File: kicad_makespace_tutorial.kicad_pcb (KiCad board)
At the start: 2 copper layers, 64.5 x 22.5 mm, 42 parts, among them J1 Screw_Terminal_01x02, J2 Conn_01x08_Pin, SW1 TS-1187A-B-A-B, SW2 TS-1187A-B-A-B, U1 AMS1117-3.3, U2 CH340C_C7464026, U3 ESP32-WROOM-32E(8MB), U4 MAX98357AETE+T

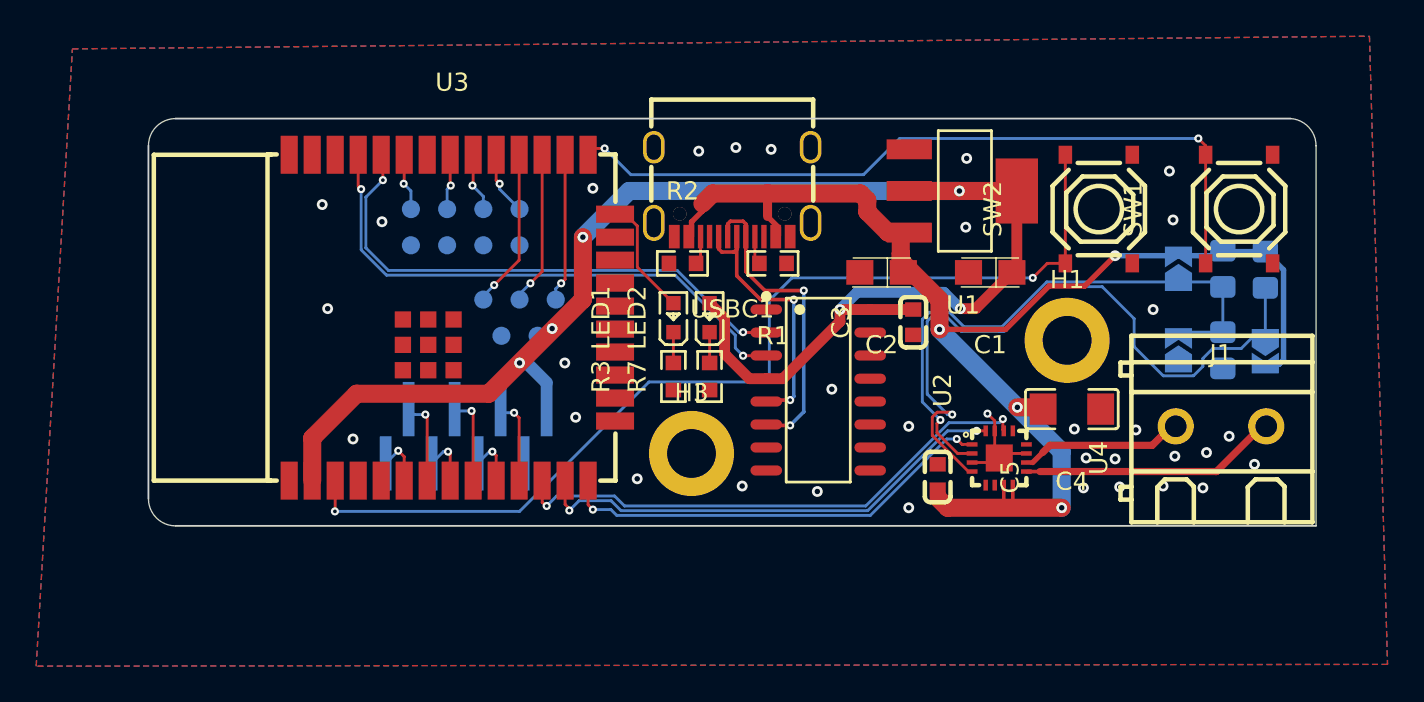
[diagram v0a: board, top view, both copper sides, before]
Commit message: Last updates
Signed-off-by: Pablo Garrido <pablogs9@gmail.com>
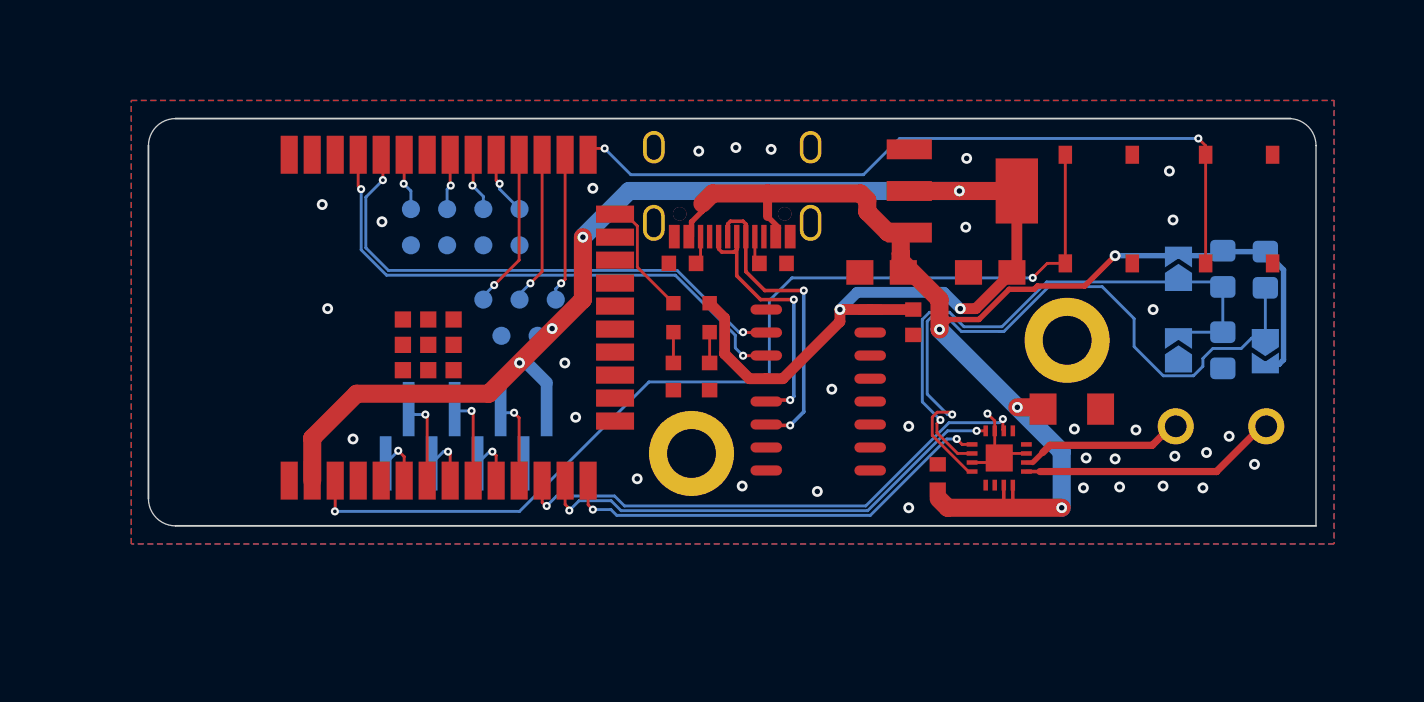
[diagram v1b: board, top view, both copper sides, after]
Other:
- board text added: "0"
- board text added: "0 mm"
- board text added: "0,01 mm"
- board text added: "0,02"
- board text added: "0,035 mm"
- board text added: "0,1600 mm / 0,1000 mm"
- board text added: "0,2000 mm"
- board text added: "1"
- board text added: "1 mm"
- board text added: "1,0900 mm"
- board text added: "2"
- board text added: "3,3"
- board text added: "4,5"
- board text added: "64,5000 mm x 22,5000 mm"
- board text added: "B.Cu"
- board text added: "B.Mask"
- board text added: "B.Paste"
- board text added: "B.Silkscreen"
- board text added: "BOARD CHARACTERISTICS"
- board text added: "Board Thickness:"
- board text added: "Board overall dimensions:"
- board text added: "Bottom Silk Screen"
- board text added: "Bottom Solder Mask"
- board text added: "Bottom Solder Paste"
- board text added: "Castellated pads:"
- board text added: "Color"
- board text added: "Copper Finish:"
- board text added: "Copper Layer Count:"
- board text added: "Dielectric 1"
- board text added: "Edge card connectors:"
- board text added: "Epsilon R"
- board text added: "F.Cu"
- board text added: "F.Mask"
- board text added: "F.Paste"
- board text added: "F.Silkscreen"
- board text added: "FR4"
- board text added: "Impedance Control:"
- board text added: "Layer Name"
- board text added: "Loss Tangent"
- board text added: "Material"
- board text added: "Min hole diameter:"
- board text added: "Min track/spacing:"
- board text added: "No"
- board text added: "None"
- board text added: "Not specified"
- board text added: "Plated Board Edge:"
- board text added: "Thickness (mm)"
- board text added: "Top Silk Screen"
- board text added: "Top Solder Mask"
- board text added: "Top Solder Paste"
- board text added: "Type"
- board text added: "copper"
- board text added: "core"

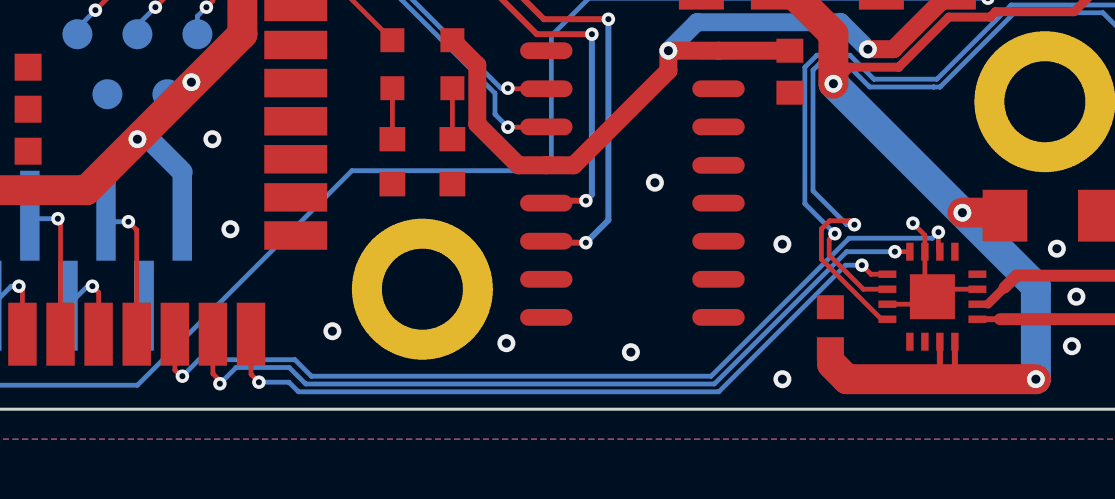
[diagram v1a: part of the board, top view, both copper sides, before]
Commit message: Minors
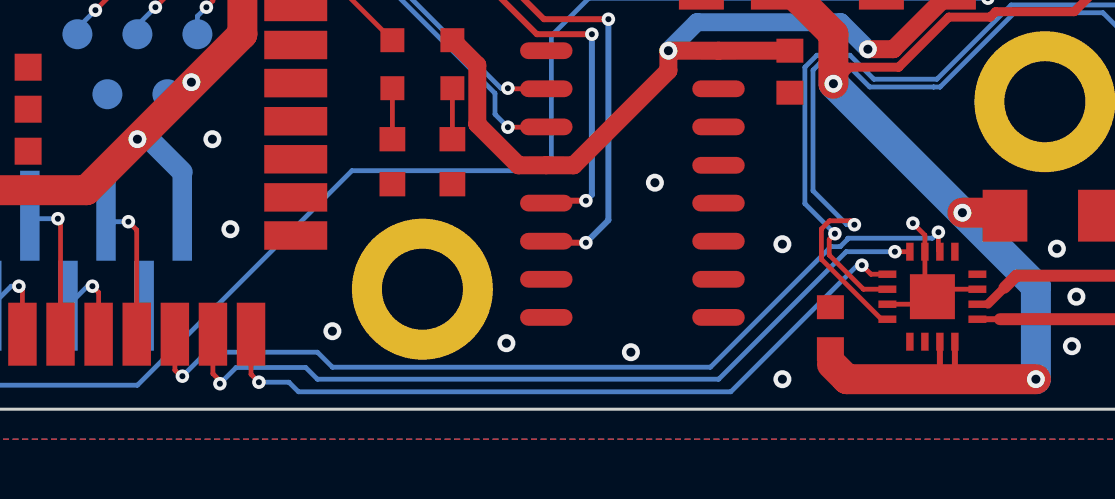
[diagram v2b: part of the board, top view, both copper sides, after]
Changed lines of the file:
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@@
-	)
-	(segment
-		(start 101.110001 121.660001)
-		(end 114.731887 121.660001)
-		(width 0.16)
-		(layer "B.Cu")
-		(net 36)
-	)
-	(segment
-		(start 119.141888 117.25)
-		(end 120.75 117.25)
-		(width 0.16)
-		(layer "B.Cu")
-		(net 36)
-	)
-	(segment
-		(start 98.79 121.11)
-		(end 100.56 121.11)
-		(width 0.16)
-		(layer "B.Cu")
-		(net 36)
-	)
-	(segment
-		(start 100.56 121.11)
-		(end 101.110001 121.660001)
-		(width 0.16)
-		(layer "B.Cu")
-		(net 36)
 	)
 	(segment
@@
 	)
 	(segment
-		(start 114.731887 121.660001)
-		(end 119.141888 117.25)
+		(start 114.875808 121.5)
+		(end 119.125808 117.25)
+		(width 0.16)
+		(layer "B.Cu")
+		(net 36)
+	)
+	(segment
+		(start 101.5 121.5)
+		(end 114.875808 121.5)
+		(width 0.16)
+		(layer "B.Cu")
+		(net 36)
+	)
+	(segment
+		(start 101.11 121.11)
+		(end 101.5 121.5)
+		(width 0.16)
+		(layer "B.Cu")
+		(net 36)
+	)
+	(segment
+		(start 119.125808 117.25)
+		(end 120.75 117.25)
+		(width 0.16)
+		(layer "B.Cu")
+		(net 36)
+	)
+	(segment
+		(start 98.79 121.11)
+		(end 101.11 121.11)
 		(width 0.16)
 		(layer "B.Cu")
@@
 	)
 	(segment
-		(start 97 121.4)
-		(end 97.55 120.85)
-		(width 0.16)
-		(layer "B.Cu")
-		(net 37)
-	)
-	(segment
-		(start 119.224192 116.8)
-		(end 122 116.8)
-		(width 0.16)
-		(layer "B.Cu")
-		(net 37)
-	)
-	(segment
-		(start 114.624192 121.4)
-		(end 119.224192 116.8)
+		(start 101.5 120.6)
+		(end 102 121.1)
 		(width 0.16)
 		(layer "B.Cu")
@@
 	)
 	(segment
-		(start 97.55 120.85)
-		(end 100.75 120.85)
-		(width 0.16)
-		(layer "B.Cu")
-		(net 37)
-	)
-	(segment
-		(start 101.3 121.4)
-		(end 114.624192 121.4)
-		(width 0.16)
-		(layer "B.Cu")
-		(net 37)
-	)
-	(segment
-		(start 100.75 120.85)
-		(end 101.3 121.4)
+		(start 114.6 121.1)
+		(end 118.62 117.08)
+		(width 0.16)
+		(layer "B.Cu")
+		(net 37)
+	)
+	(segment
+		(start 119.18 116.828112)
+		(end 119.18 116.8)
+		(width 0.16)
+		(layer "B.Cu")
+		(net 37)
+	)
+	(segment
+		(start 97 121.4)
+		(end 97.8 120.6)
+		(width 0.16)
+		(layer "B.Cu")
+		(net 37)
+	)
+	(segment
+		(start 97.8 120.6)
+		(end 101.5 120.6)
+		(width 0.16)
+		(layer "B.Cu")
+		(net 37)
+	)
+	(segment
+		(start 118.62 117.08)
+		(end 118.928112 117.08)
+		(width 0.16)
+		(layer "B.Cu")
+		(net 37)
+	)
+	(segment
+		(start 102 121.1)
+		(end 114.6 121.1)
+		(width 0.16)
+		(layer "B.Cu")
+		(net 37)
+	)
+	(segment
+		(start 118.928112 117.08)
+		(end 119.18 116.828112)
+		(width 0.16)
+		(layer "B.Cu")
+		(net 37)
+	)
+	(segment
+		(start 119.18 116.8)
+		(end 122 116.8)
 		(width 0.16)
 		(layer "B.Cu")
@@
 	)
 	(segment
-		(start 114.88 121.92)
-		(end 119.1 117.7)
-		(width 0.16)
-		(layer "B.Cu")
-		(net 41)
-	)
-	(segment
 		(start 100.55 121.6)
 		(end 100.87 121.92)
@@
 	)
 	(segment
+		(start 100.87 121.92)
+		(end 115.28 121.92)
+		(width 0.16)
+		(layer "B.Cu")
+		(net 41)
+	)
+	(segment
+		(start 115.28 121.92)
+		(end 119.5 117.7)
+		(width 0.16)
+		(layer "B.Cu")
+		(net 41)
+	)
+	(segment
 		(start 99.55 121.6)
 		(end 100.55 121.6)
@@
 	)
 	(segment
-		(start 119.1 117.7)
+		(start 119.5 117.7)
 		(end 119.65 117.7)
 		(width 0.16)
 		(layer "B.Cu")
-		(net 41)
-	)
-	(segment
-		(start 100.87 121.92)
-		(end 114.88 121.92)
-		(width 0.16)
-		(layer "B.Cu")
